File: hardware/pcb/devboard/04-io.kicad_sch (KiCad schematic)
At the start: 13 parts, among them J13 CLAVIER INTERNE, J6 USB-C CHARGE + PROG, J7 USB-C CLAVIER (hote), J8 microSD

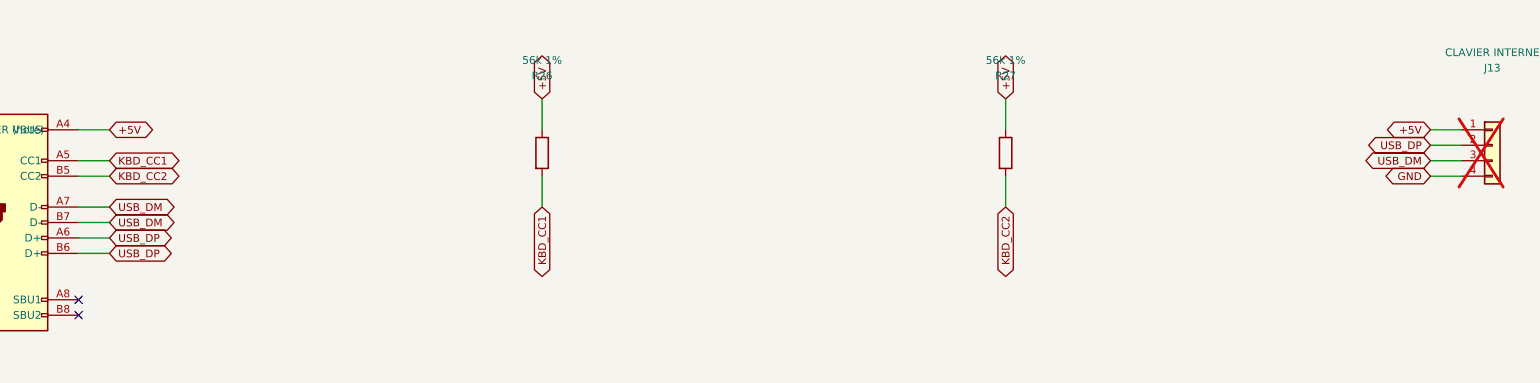
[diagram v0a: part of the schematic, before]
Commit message: Update mainboard
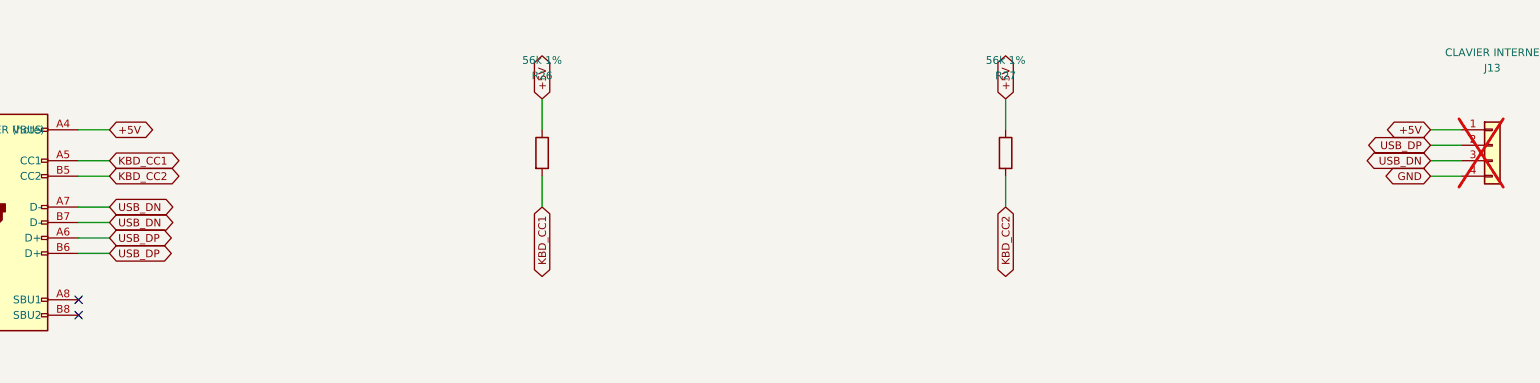
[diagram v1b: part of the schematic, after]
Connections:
- net USB_DM renamed USB_DN
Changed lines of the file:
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@@
 		)
 	)
-	(global_label "USB_DM"
+	(global_label "USB_DN"
 		(shape bidirectional)
 		(at 342.9 69.85 0)
@@
 		)
 	)
-	(global_label "USB_DM"
+	(global_label "USB_DN"
 		(shape bidirectional)
 		(at 342.9 72.39 0)
@@
 		)
 	)
-	(global_label "USB_DM"
+	(global_label "USB_DN"
 		(shape bidirectional)
 		(at 560.0699999999999 62.23 180)
